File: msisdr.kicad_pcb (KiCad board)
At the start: 2 copper layers, 46.3 x 90.7 mm, 82 parts, among them J1 VCC_GPIO, J10 SMA_VHF1, J11 USB_OTG, J2 GPIO0, J3 GPIO1, J4 GPIO2, J5 GPIO3, J6 SMA_0_30MHZ, J7 SMA_30_60MHZ, J8 SMA_VHF2, J9 SMA_UHF, U1 msi2500, U2 msi001, U3 RT9193-28, U4 AP7313-30SAG, Y1 24MHz, Y2 24MHZ

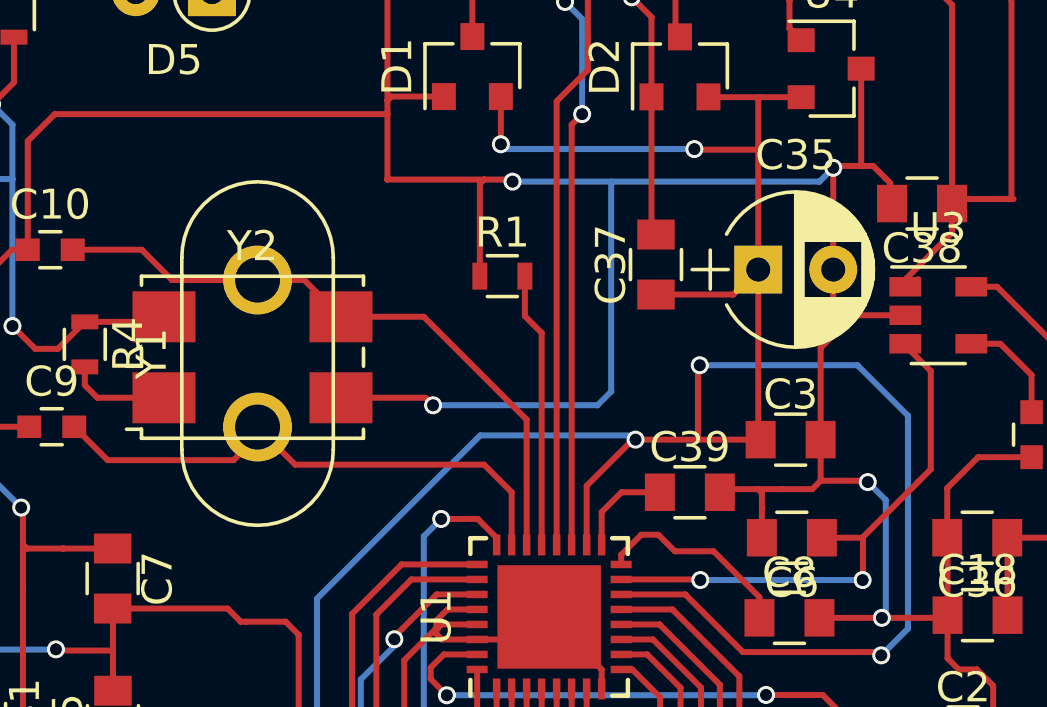
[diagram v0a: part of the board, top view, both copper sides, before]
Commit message: converted to kicad 6.0 project
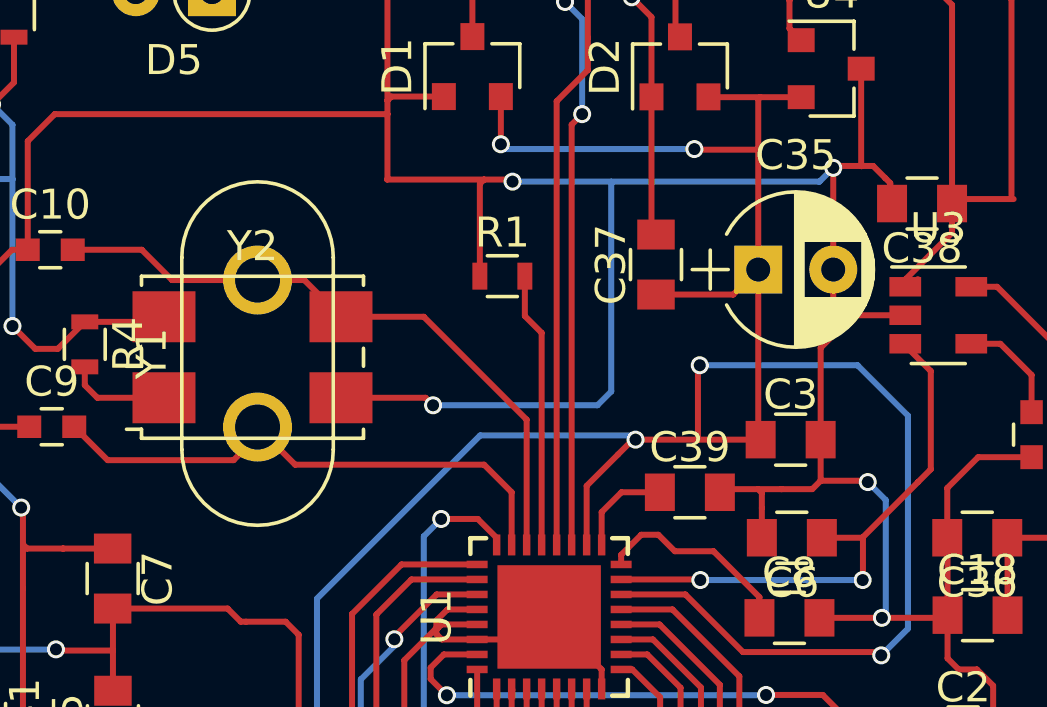
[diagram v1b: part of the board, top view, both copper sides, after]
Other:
- net class Default removed
- net class GND removed
- net class VDIG removed
- net class VRF removed
